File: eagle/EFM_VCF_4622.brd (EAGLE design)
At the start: 102.1 x 80.8 mm, 57 parts, among them IC1 LM13700N, Q1 2N3906, Q10 2N3904, Q11 2N3904, Q12 2N3904, Q13 2N3904, Q2 2N3904, Q3 2N3904, Q4 2N3904, Q5 2N3904, Q6 2N3904, Q7 2N3904, Q8 2N3904, Q9 2N3904

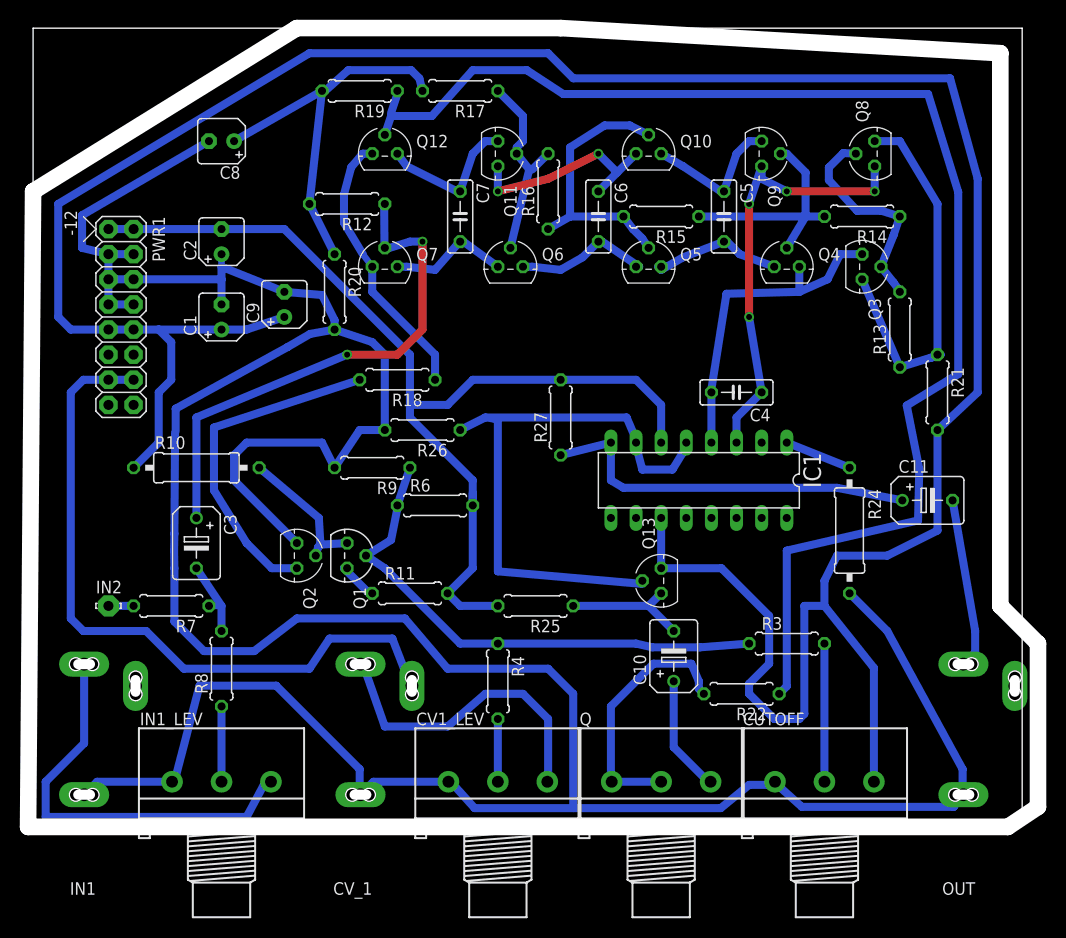
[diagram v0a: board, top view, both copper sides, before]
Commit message: ready to cut
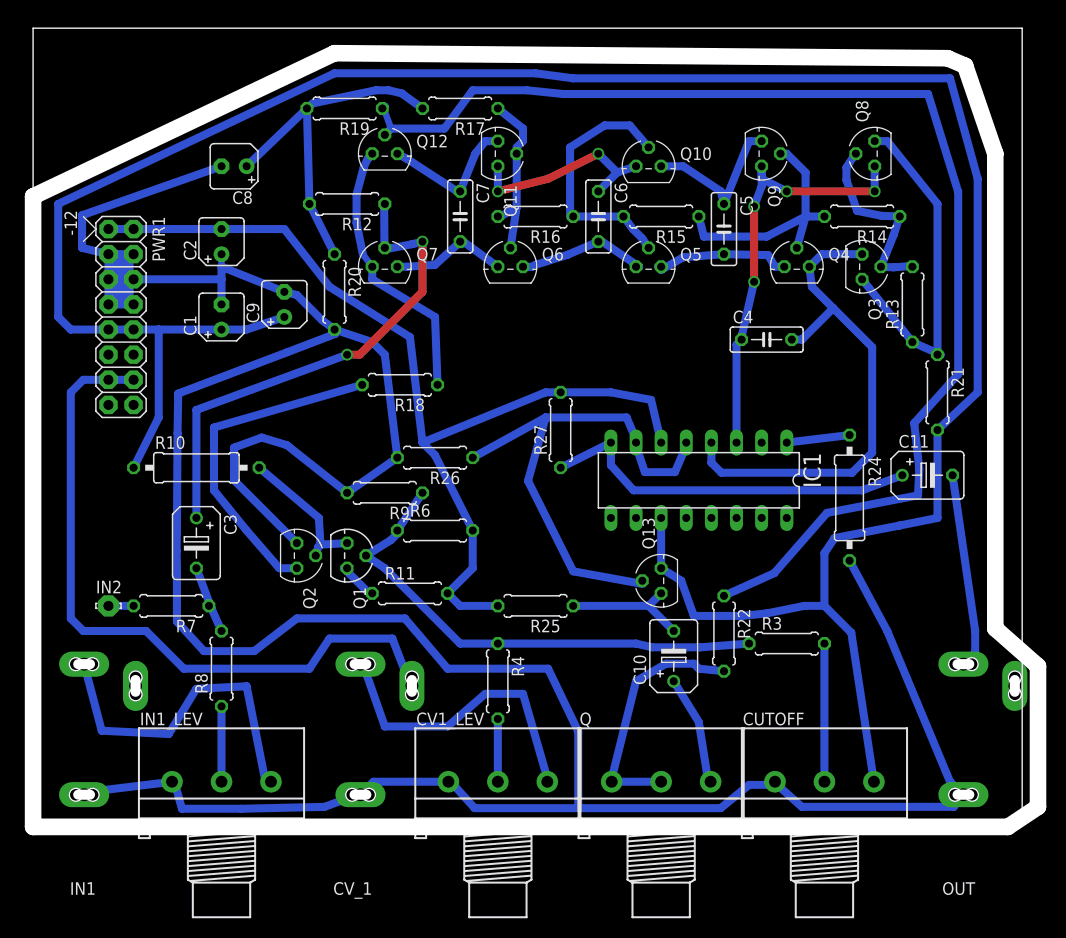
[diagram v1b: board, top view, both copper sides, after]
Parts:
- moved R22 6.35 mm to (69.8, 18.8), turned to 270 degrees
- moved C4 6.14 mm to (74.2, 48.5), turned to 0 degrees
- moved R24 3.30 mm to (82.5, 32.5)
- moved R26 3.07 mm to (40.6, 36.6)
- moved R13 2.84 mm to (88.9, 52.1)
- moved R16 2.84 mm to (50.8, 61.0), turned to 180 degrees
- moved R9 2.84 mm to (35.6, 33.0)
- moved C8 2.84 mm to (20.3, 66.0)
- moved C11 2.54 mm to (90.4, 34.8)
- moved R6 2.54 mm to (40.6, 29.2)
- moved R19 2.34 mm to (31.5, 71.9)
- moved R17 1.78 mm to (43.2, 71.9)
- moved C5 1.27 mm to (69.8, 59.7)
- moved R27 1.27 mm to (53.3, 39.4)
- moved Q10 1.27 mm to (62.2, 66.0)
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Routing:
- net +12V: track 276.6 -> 250.7 mm
- net N$9: track 33.3 -> 52.3 mm
- net N$26: track 136.8 -> 125.7 mm
- net N$58: track 42.0 -> 34.6 mm
- net N$19: track 60.4 -> 53.0 mm
- net GND: track 335.1 -> 329.2 mm
- net -12V: track 101.7 -> 97.5 mm
- net N$43: track 40.2 -> 36.1 mm
- net N$25: track 39.7 -> 36.3 mm
- net N$50: track 20.4 -> 17.8 mm
- net N$31: track 17.2 -> 19.8 mm
- net N$44: track 21.9 -> 19.4 mm
- net N$7: track 53.1 -> 51.3 mm
- net N$20: track 52.9 -> 51.1 mm
- net N$49: track 27.8 -> 26.1 mm
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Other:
- board size 102.1 x 80.8 mm -> 101.6 x 80.8 mm
